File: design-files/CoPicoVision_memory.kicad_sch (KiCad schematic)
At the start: 13 parts, among them U103 74ACT05, U201 GAL22V10, U202 GAL22V10, U203 AT28C64, U204 AS6C62256, U205 74HCT08, U206 74HCT74

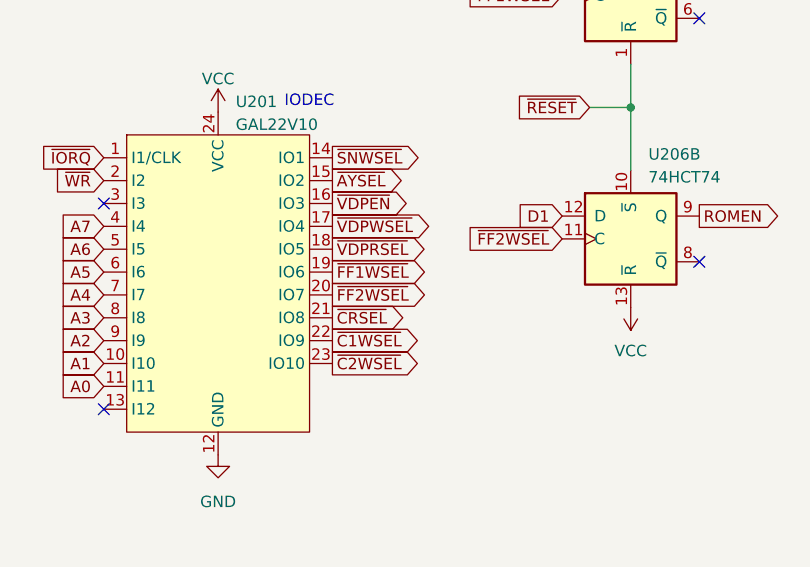
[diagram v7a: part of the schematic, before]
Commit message: Route most of the address / data lines.
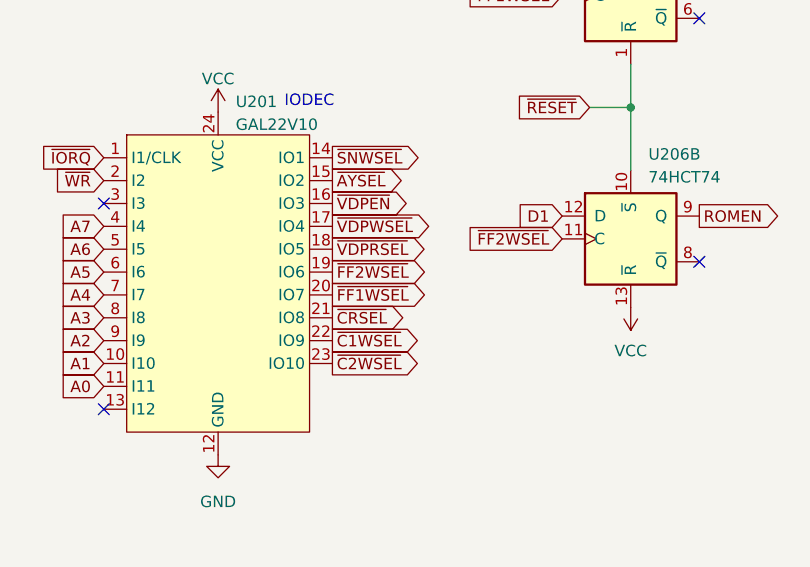
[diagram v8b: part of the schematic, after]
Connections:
- net ~{FF1WSEL}: now also U201.20 (IO7); no longer U201.19 (IO6)
- net ~{FF2WSEL}: now also U201.19 (IO6); no longer U201.20 (IO7)
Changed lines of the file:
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@@
     )
   )
-  (global_label "~{FF2WSEL}" (shape output) (at 121.158 62.992 0) (fields_autoplaced)
+  (global_label "~{FF2WSEL}" (shape output) (at 121.158 60.452 0) (fields_autoplaced)
     (effects (font (size 1.27 1.27)) (justify left))
-    (property "Intersheetrefs" "${INTERSHEET_REFS}" (at 132.2885 62.992 0)
+    (property "Intersheetrefs" "${INTERSHEET_REFS}" (at 132.2885 60.452 0)
       (effects (font (size 1.27 1.27)) (justify left) hide)
     )
@@
     )
   )
-  (global_label "~{FF1WSEL}" (shape output) (at 121.158 60.452 0) (fields_autoplaced)
+  (global_label "~{FF1WSEL}" (shape output) (at 121.158 62.992 0) (fields_autoplaced)
     (effects (font (size 1.27 1.27)) (justify left))
-    (property "Intersheetrefs" "${INTERSHEET_REFS}" (at 132.2885 60.452 0)
+    (property "Intersheetrefs" "${INTERSHEET_REFS}" (at 132.2885 62.992 0)
       (effects (font (size 1.27 1.27)) (justify left) hide)
     )
